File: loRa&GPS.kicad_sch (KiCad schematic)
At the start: 13 parts, among them J4 Conn_Coaxial, U10 RAK3172, U3 STA8135GA, U9 TESEO-LIV4F

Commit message: lib allign
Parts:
- BT1: footprint (none) -> Battery:BatteryHolder_Seiko_MS621F
- D8: footprint (none) -> Diode_SMD:D_0603_1608Metric_Pad1.05x0.95mm_HandSolder
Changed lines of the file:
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@@
 			)
 		)
-		(property "Footprint" ""
+		(property "Footprint" "Battery:BatteryHolder_Seiko_MS621F"
 			(at 99.568 46.228 90)
 			(effects
@@
 			)
 		)
-		(property "Footprint" ""
+		(property "Footprint" "Diode_SMD:D_0603_1608Metric_Pad1.05x0.95mm_HandSolder"
 			(at 99.568 25.654 90)
 			(effects

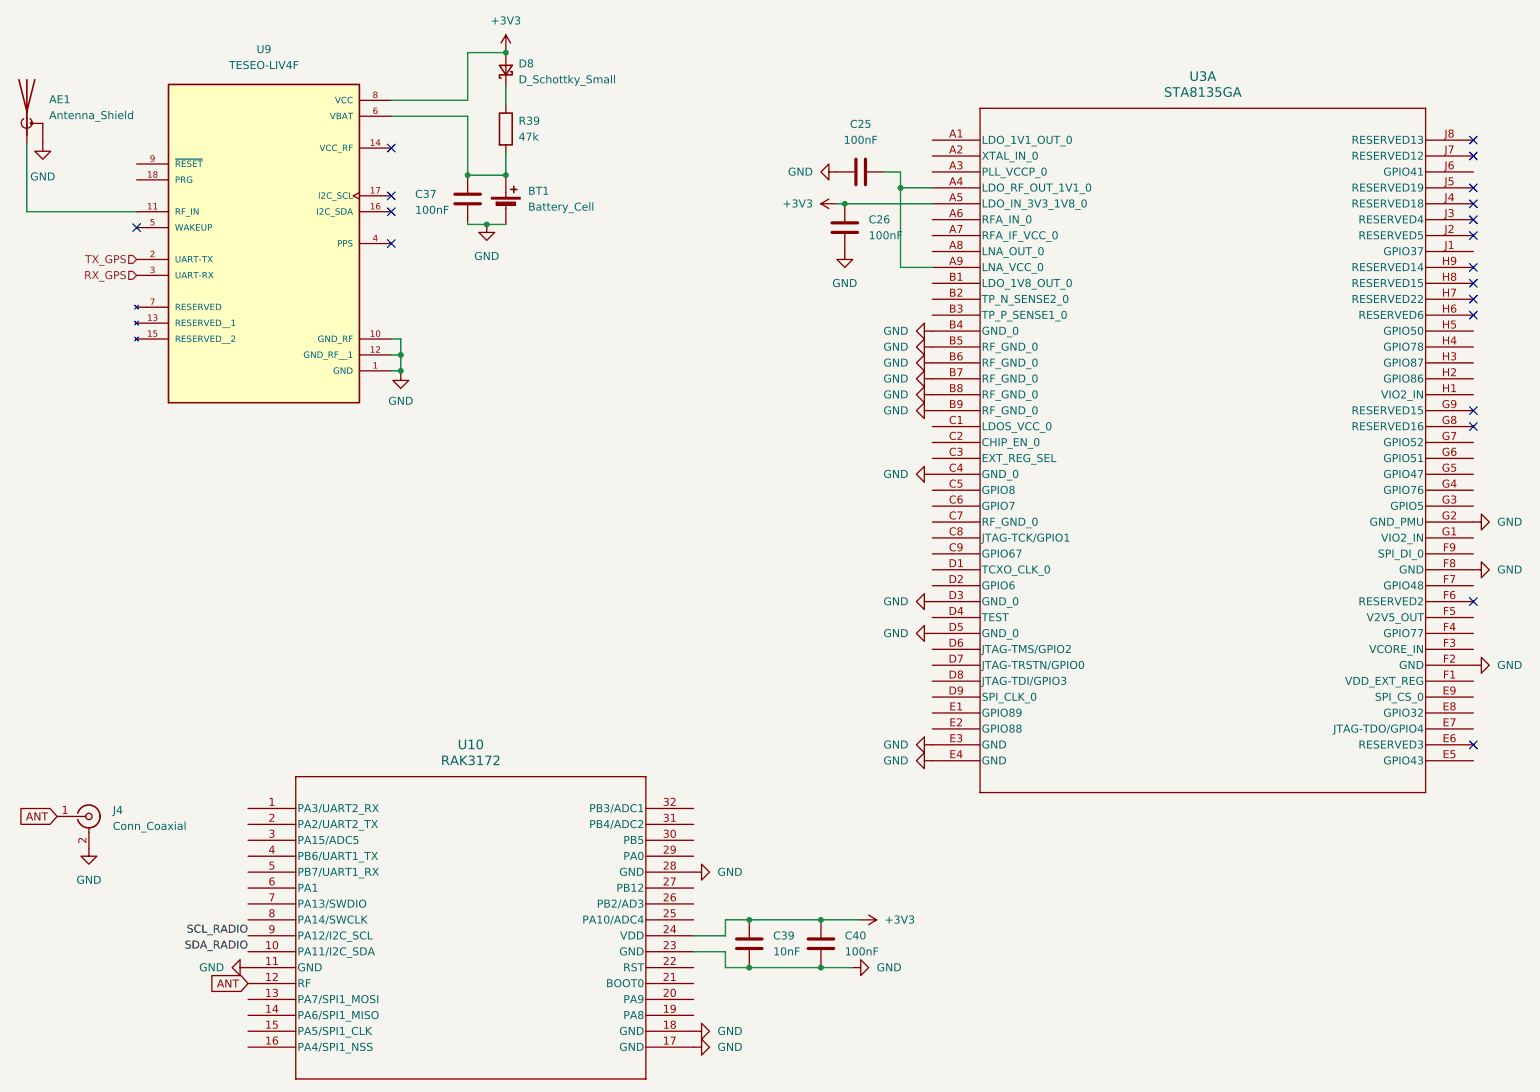
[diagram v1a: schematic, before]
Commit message: Aggiornamento routing
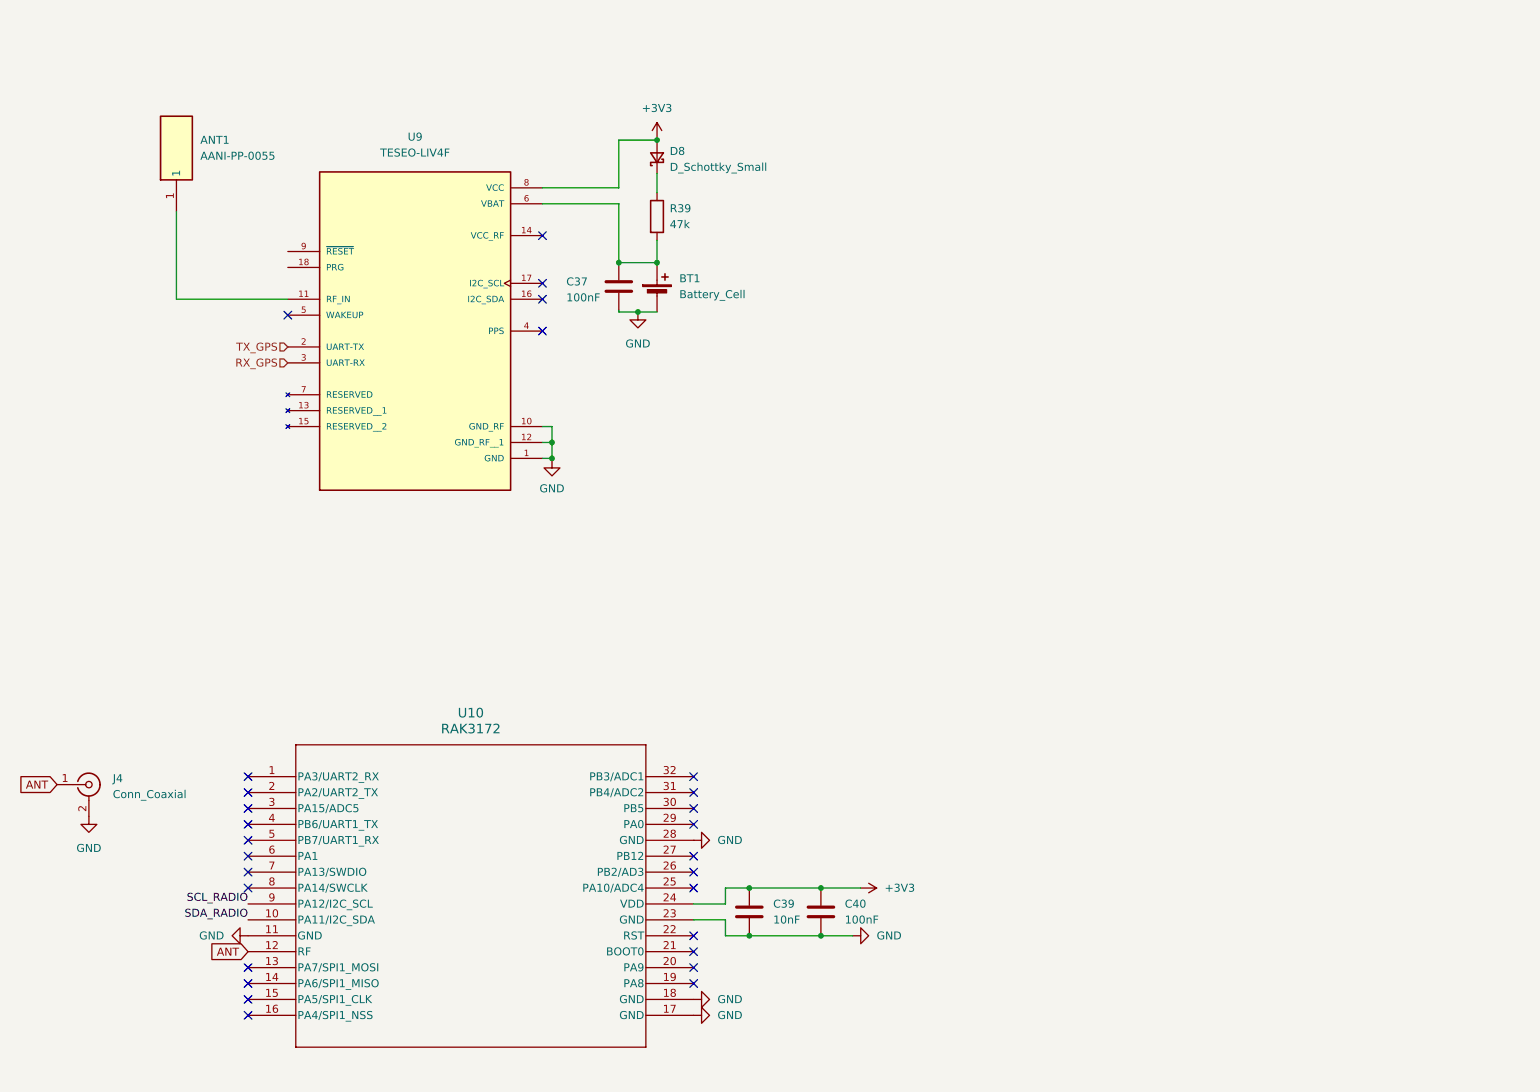
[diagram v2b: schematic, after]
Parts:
- removed AE1: Antenna_Shield, symbol Device:Antenna_Shield
- removed C25, C26: 100nF, Capacitor_SMD:C_0603_1608Metric_Pad1.08x0.95mm_HandSolder, symbol Device:C
- removed U3: STA8135GA, footprints:TFBGA160_7X11X1p2_STM, symbol 2025-11-15_15-30-48:STA8135GA
- added ANT1: AANI-PP-0055, AANIPP0055, symbol AANI-PP-0055:AANI-PP-0055
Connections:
- net at U9.11 (RF_IN): now also ANT1.1
- no-connect marks 19 -> 28
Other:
- moved on the sheet: BT1, C37, C39, C40, D8, J4, R39, U10, U9

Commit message: fix continuo
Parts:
- ANT1: footprint AANIPP0055 -> antenna_GPS:AANIPP0055
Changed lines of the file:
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@@
 			)
 		)
-		(property "Footprint" "AANIPP0055"
+		(property "Footprint" "antenna_GPS:AANIPP0055"
 			(at 141.91 31.75 0)
 			(effects
